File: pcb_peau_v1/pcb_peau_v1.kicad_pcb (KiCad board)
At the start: 2 copper layers, 70 x 70 mm, 26 parts, among them J1 Conn_01x05, J2 Conn_01x05, J4 Conn_02x08_Top_Bottom, J5 Conn_02x12_Top_Bottom, U2 TLC274, U3 CD74HC4067SM, U4 CD74HC4067SM, U5 CD74HC4067SM, U6 CD74HC4067SM, U7 TLC274, U8 TLC274, U9 TLC274

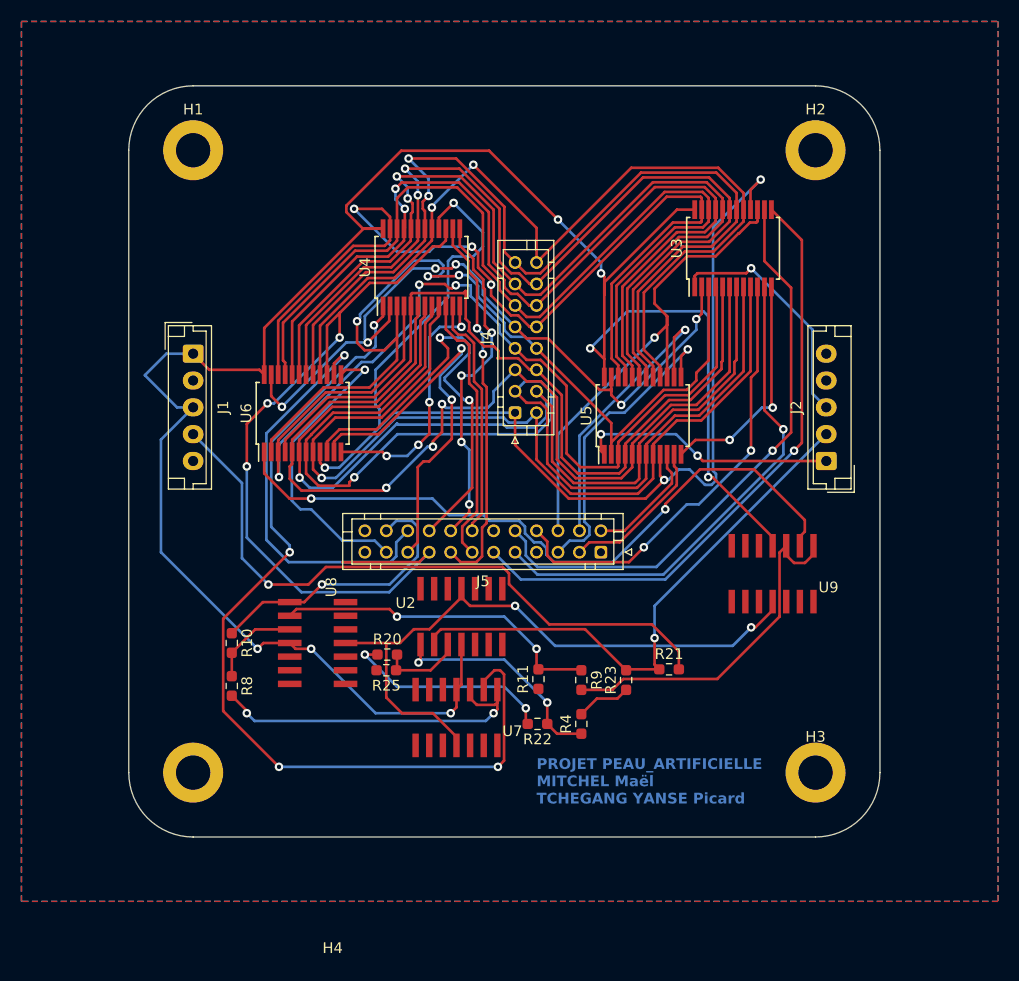
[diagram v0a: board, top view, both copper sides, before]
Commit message: Pcb Corrigé presque pret
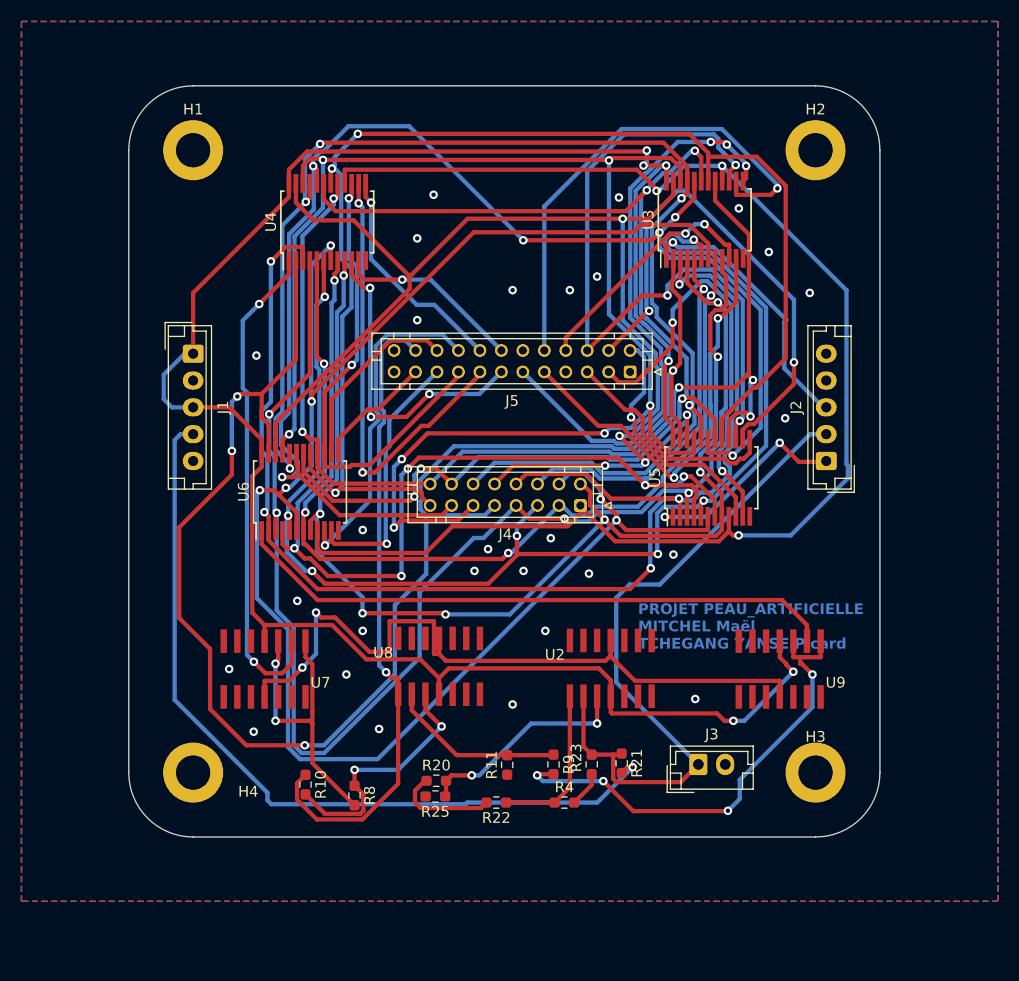
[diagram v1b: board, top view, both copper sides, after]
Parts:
- added J3: Conn_01x02, Connector_JST:JST_EH_B2B-EH-A_1x02_P2.50mm_Vertical, F.Cu at (225.1, 110.2)
- moved U7 18.4 mm to (184.7, 101.3)
- moved J5 17.0 mm to (218.7, 73.7)
- moved R8 15.3 mm to (193.0, 113.1)
- moved R10 14.9 mm to (188.5, 112.1)
- moved U2 14.7 mm to (216.9, 101.3)
- moved R20 12.6 mm to (200.7, 111.8)
- moved R25 12.6 mm to (200.6, 113.2)
- moved U8 11.5 mm to (200.9, 101.1), turned to 0 degrees
- moved J4 10.6 mm to (214.1, 86.1), turned to 180 degrees
- moved R21 9.81 mm to (217.9, 110.1), turned to -90 degrees
- moved U4 9.74 mm to (190.5, 59.7)
- moved U9 8.91 mm to (232.7, 101.3)
- moved U5 8.63 mm to (226.3, 83.5)
- moved R11 8.51 mm to (207.3, 110.3)
- moved R23 8.49 mm to (215.1, 110.2)
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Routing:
- net Net-(J4-Pin_9): track 68.5 -> 150.2 mm, vias 6 -> 4
- net Net-(J4-Pin_4): track 91.9 -> 163.2 mm, vias 1 -> 6
- net Net-(J4-Pin_11): track 87.6 -> 141.3 mm, vias 0 -> 7
- net 0: track 45.3 -> 0.00 mm, vias 6 -> 27
- net Net-(J4-Pin_8): track 86.7 -> 128.3 mm, vias 3 -> 5
- net Net-(J4-Pin_6): track 77.2 -> 118.2 mm, vias 0 -> 6
- net Net-(J4-Pin_13): track 90.1 -> 130.3 mm, vias 2 -> 6
- net AOP1: track 85.8 -> 46.0 mm, vias 4 -> 2
- net Net-(J4-Pin_12): track 89.0 -> 125.8 mm, vias 2 -> 5
- net TRIOAOP1: track 26.6 -> 60.0 mm
- net Net-(J4-Pin_15): track 92.3 -> 122.4 mm, vias 2 -> 3
- net NE2: track 74.1 -> 44.6 mm, vias 3 -> 2
- net Net-(J4-Pin_7): track 99.9 -> 129.3 mm, vias 3 -> 5
- net Net-(J4-Pin_5): track 93.3 -> 121.5 mm, vias 3 -> 7
- net Net-(J4-Pin_10): track 90.4 -> 116.2 mm, vias 3 -> 5
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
